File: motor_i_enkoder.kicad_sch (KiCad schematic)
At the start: 13 parts, among them J7 Conn_02x06_Odd_Even, M1 Motor_DC, SW2 RotaryEncoder, U4 L298N

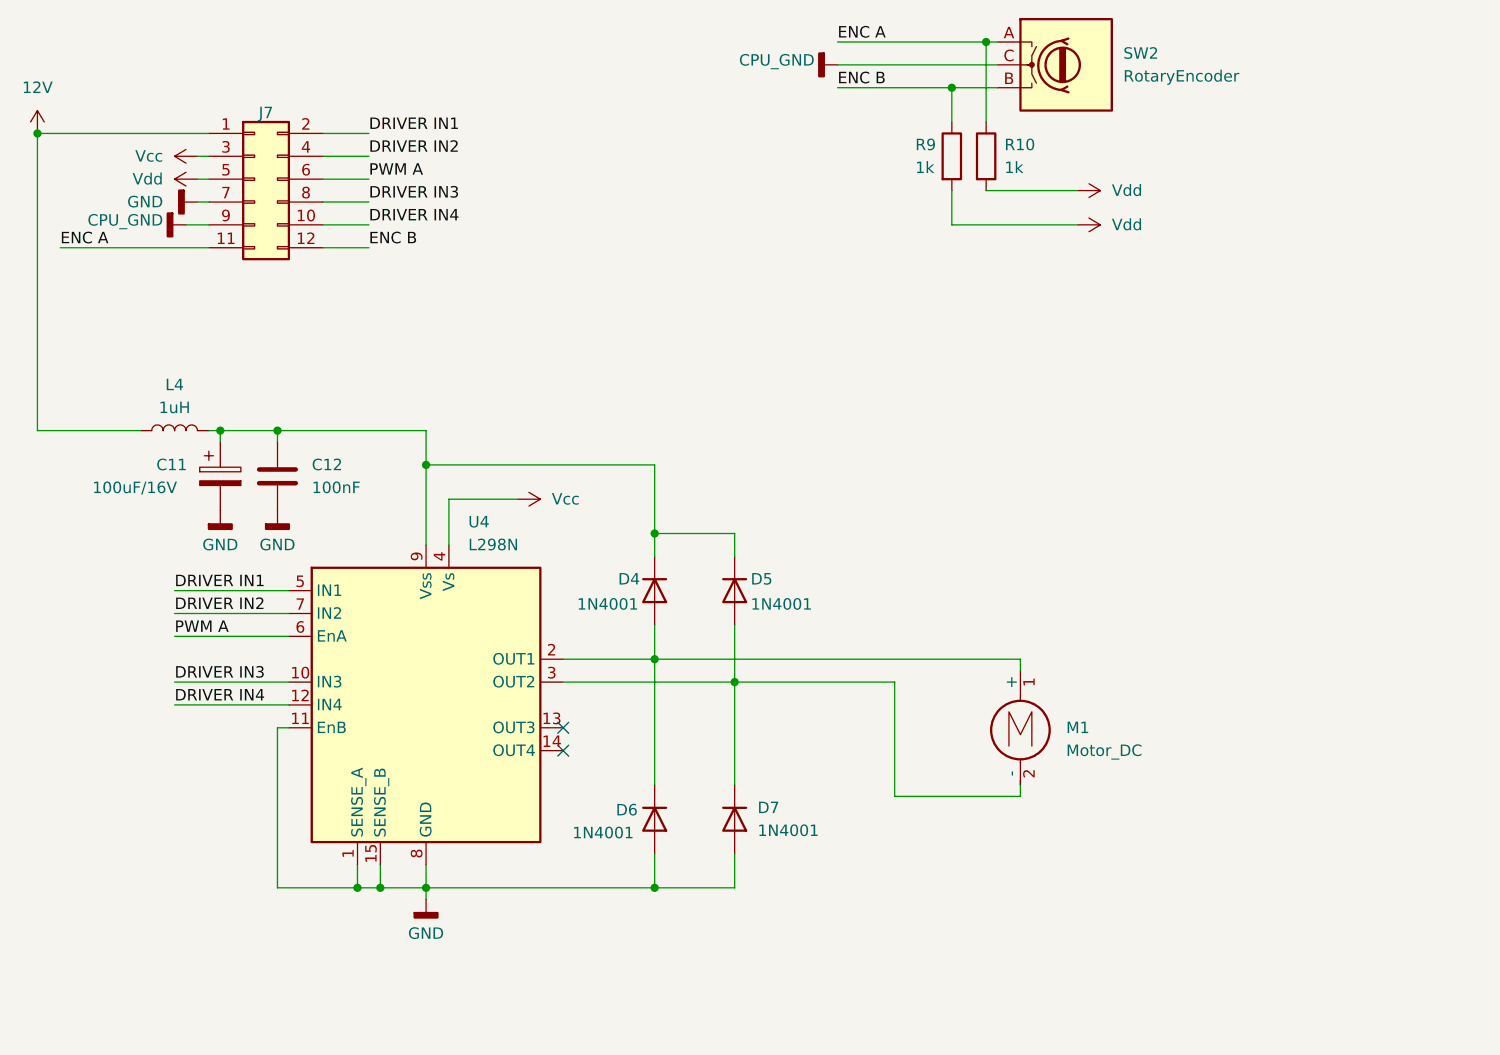
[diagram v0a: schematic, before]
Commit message: Niedziela
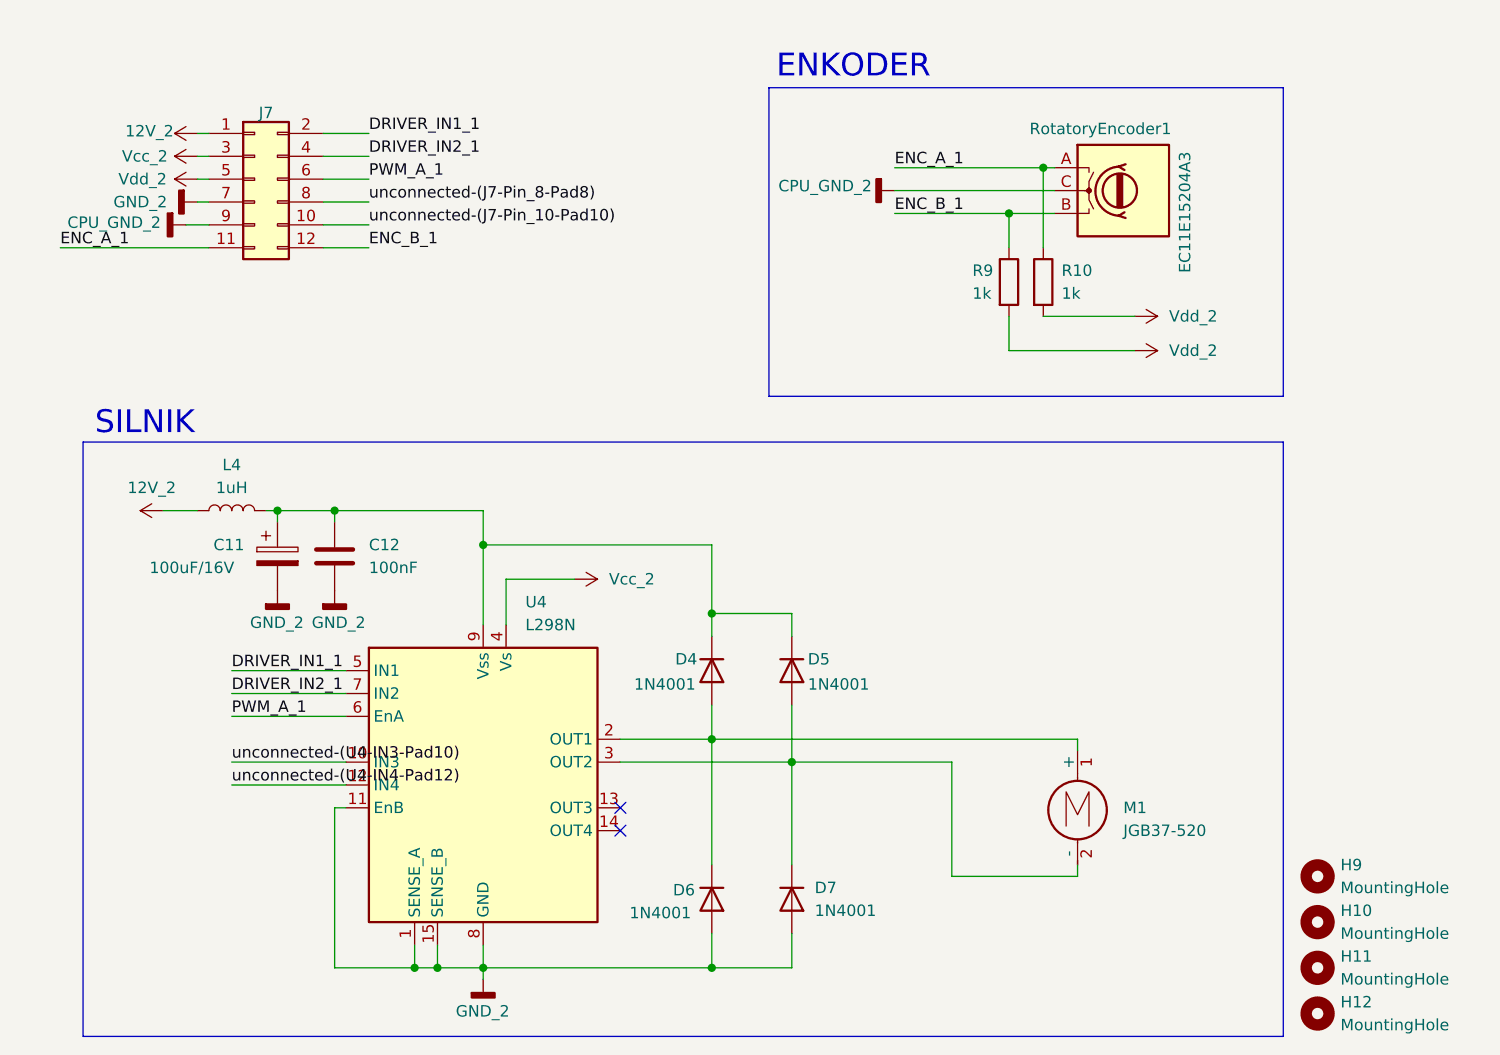
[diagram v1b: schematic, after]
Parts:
- added H10, H11, H12, H9: MountingHole, MountingHole:MountingHole_3.2mm_M3_DIN965_Pad_TopBottom, symbol Mechanical:MountingHole
- C11: footprint (none) -> Capacitor_SMD:C_Elec_6.3x7.7; KiLib_Generator (none) -> capacitor/THT/other
- C12: footprint (none) -> Capacitor_SMD:C_0805_2012Metric_Pad1.18x1.45mm_HandSolder; KiLib_Generator (none) -> SMD_2terminal_chip_molded
- D4, D5, D6, D7: footprint (none) -> Diode_SMD:D_SMA; KiLib_Generator (none) -> diode/THT
- J7: footprint (none) -> Connector_PinHeader_2.54mm:PinHeader_2x06_P2.54mm_Vertical; KiLib_Generator (none) -> connector/pin_header_socket
- L4: footprint (none) -> Inductor_SMD:L_Bourns_SRR1260; KiLib_Generator (none) -> SMD_2terminal_chip_molded
- M1: value Motor_DC -> JGB37-520; footprint (none) -> TerminalBlock_MetzConnect:TerminalBlock_MetzConnect_Type011_RT05502HBLC_1x02_P5.00mm_Horizontal; KiLib_Generator (none) -> terminal_block/Metz_Connect
- R10, R9: footprint (none) -> Resistor_SMD:R_1206_3216Metric_Pad1.30x1.75mm_HandSolder; KiLib_Generator (none) -> SMD_2terminal_chip_molded
- RotatoryEncoder1: renamed from SW2; value RotaryEncoder -> EC11E15204A3; footprint (none) -> Rotary_Encoder:RotaryEncoder_Alps_EC11E_Vertical_H20mm
- U4: KiLib_Generator (none) -> package/TO_SOT/THT
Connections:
- net 12V renamed 12V_2
- net CPU_GND renamed CPU_GND_2
- net DRIVER IN1 renamed DRIVER_IN1_1
- net DRIVER IN2 renamed DRIVER_IN2_1
- net DRIVER IN3 renamed unconnected-(J7-Pin_8-Pad8)
- net unconnected-(J7-Pin_8-Pad8): no longer U4.10 (IN3)
- net DRIVER IN4 renamed unconnected-(J7-Pin_10-Pad10)
- net unconnected-(J7-Pin_10-Pad10): no longer U4.12 (IN4)
- net ENC A renamed ENC_A_1
- net ENC B renamed ENC_B_1
- net GND renamed GND_2
- net PWM A renamed PWM_A_1
- net Vcc renamed Vcc_2
- net Vdd renamed Vdd_2
- new net unconnected-(U4-IN3-Pad10): U4.10 (IN3)
- new net unconnected-(U4-IN4-Pad12): U4.12 (IN4)
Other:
- note added: "ENKODER"
- note added: "SILNIK"
- moved on the sheet: C11, C12, D4, D5, D6, D7, L4, R10, R9, RotatoryEncoder1, U4
